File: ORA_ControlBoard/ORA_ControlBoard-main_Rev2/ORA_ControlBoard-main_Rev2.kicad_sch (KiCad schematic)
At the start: 66 parts, among them J1 SM04B-GHS-TB, J2 Conn_01x04_Pin, J3 USB_B_Micro, J4 12V, J5 SM04B-GHS-TB, J6 Conn_02x03_Top_Bottom, J7 Conn_01x05_Pin, J8 Conn_01x05_Pin, J9 Stack Light, Q1 BS170, Q3 BS170, Q5 BS170, SW1 Reset, U1 ATmega32U4-A, U2 MCP25625-x-SS, U5 NCP1117-5.0_SOT223, U6 IMU_MOUNT, Y1 8Mhz, Y2 16MHz

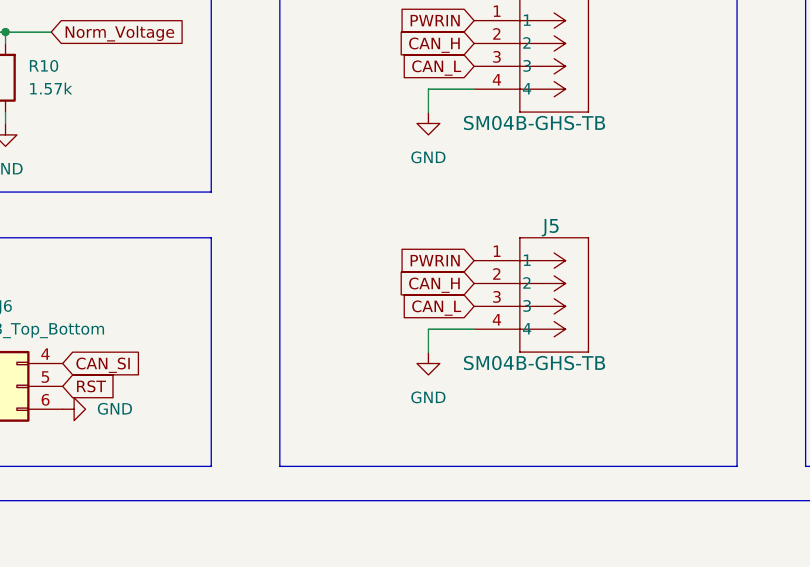
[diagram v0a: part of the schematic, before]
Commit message: Fixed Spring Cleaning
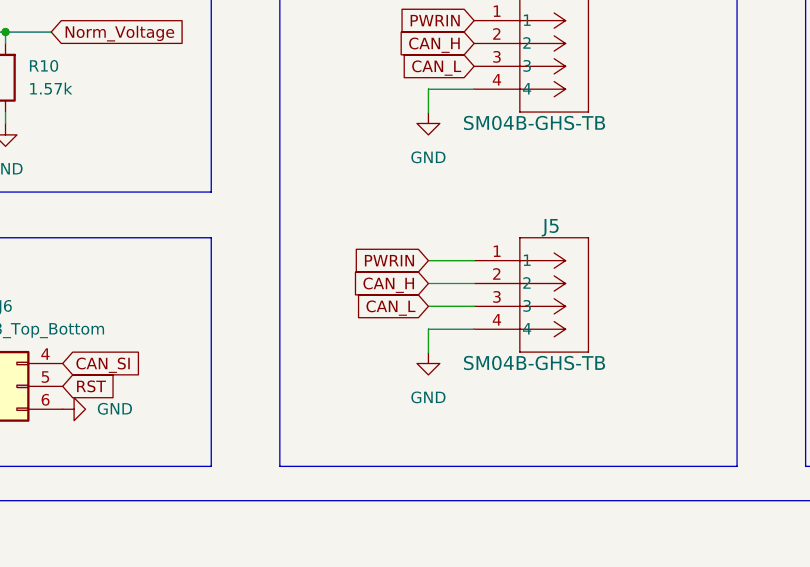
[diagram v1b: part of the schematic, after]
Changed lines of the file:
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@@
 	(wire
 		(pts
+			(xy 187.96 140.97) (xy 193.04 140.97)
+		)
+		(stroke
+			(width 0)
+			(type default)
+		)
+	)
+	(wire
+		(pts
 			(xy 287.02 101.6) (xy 280.67 101.6)
 		)
@@
 	(wire
 		(pts
+			(xy 187.96 138.43) (xy 193.04 138.43)
+		)
+		(stroke
+			(width 0)
+			(type default)
+		)
+	)
+	(wire
+		(pts
 			(xy 54.61 213.36) (xy 54.61 214.63)
 		)
@@
 	(wire
 		(pts
+			(xy 187.96 135.89) (xy 193.04 135.89)
+		)
+		(stroke
+			(width 0)
+			(type default)
+		)
+	)
+	(wire
+		(pts
 			(xy 266.7 78.74) (xy 262.89 78.74)
 		)
@@
 	(global_label "PWRIN"
 		(shape input)
-		(at 193.04 135.89 180)
+		(at 187.96 135.89 180)
 		(fields_autoplaced yes)
 		(effects
@@
 		)
 		(property "Intersheetrefs" "${INTERSHEET_REFS}"
-			(at 184.1281 135.89 0)
+			(at 179.0481 135.89 0)
 			(effects
 				(font
@@
 	(global_label "CAN_L"
 		(shape input)
-		(at 193.04 140.97 180)
+		(at 187.96 140.97 180)
 		(fields_autoplaced yes)
 		(effects
@@
 		)
 		(property "Intersheetrefs" "${INTERSHEET_REFS}"
-			(at 184.37 140.97 0)
+			(at 179.29 140.97 0)
 			(effects
 				(font
@@
 	(global_label "CAN_H"
 		(shape input)
-		(at 193.04 138.43 180)
+		(at 187.96 138.43 180)
 		(fields_autoplaced yes)
 		(effects
@@
 		)
 		(property "Intersheetrefs" "${INTERSHEET_REFS}"
-			(at 184.0676 138.43 0)
+			(at 178.9876 138.43 0)
 			(effects
 				(font

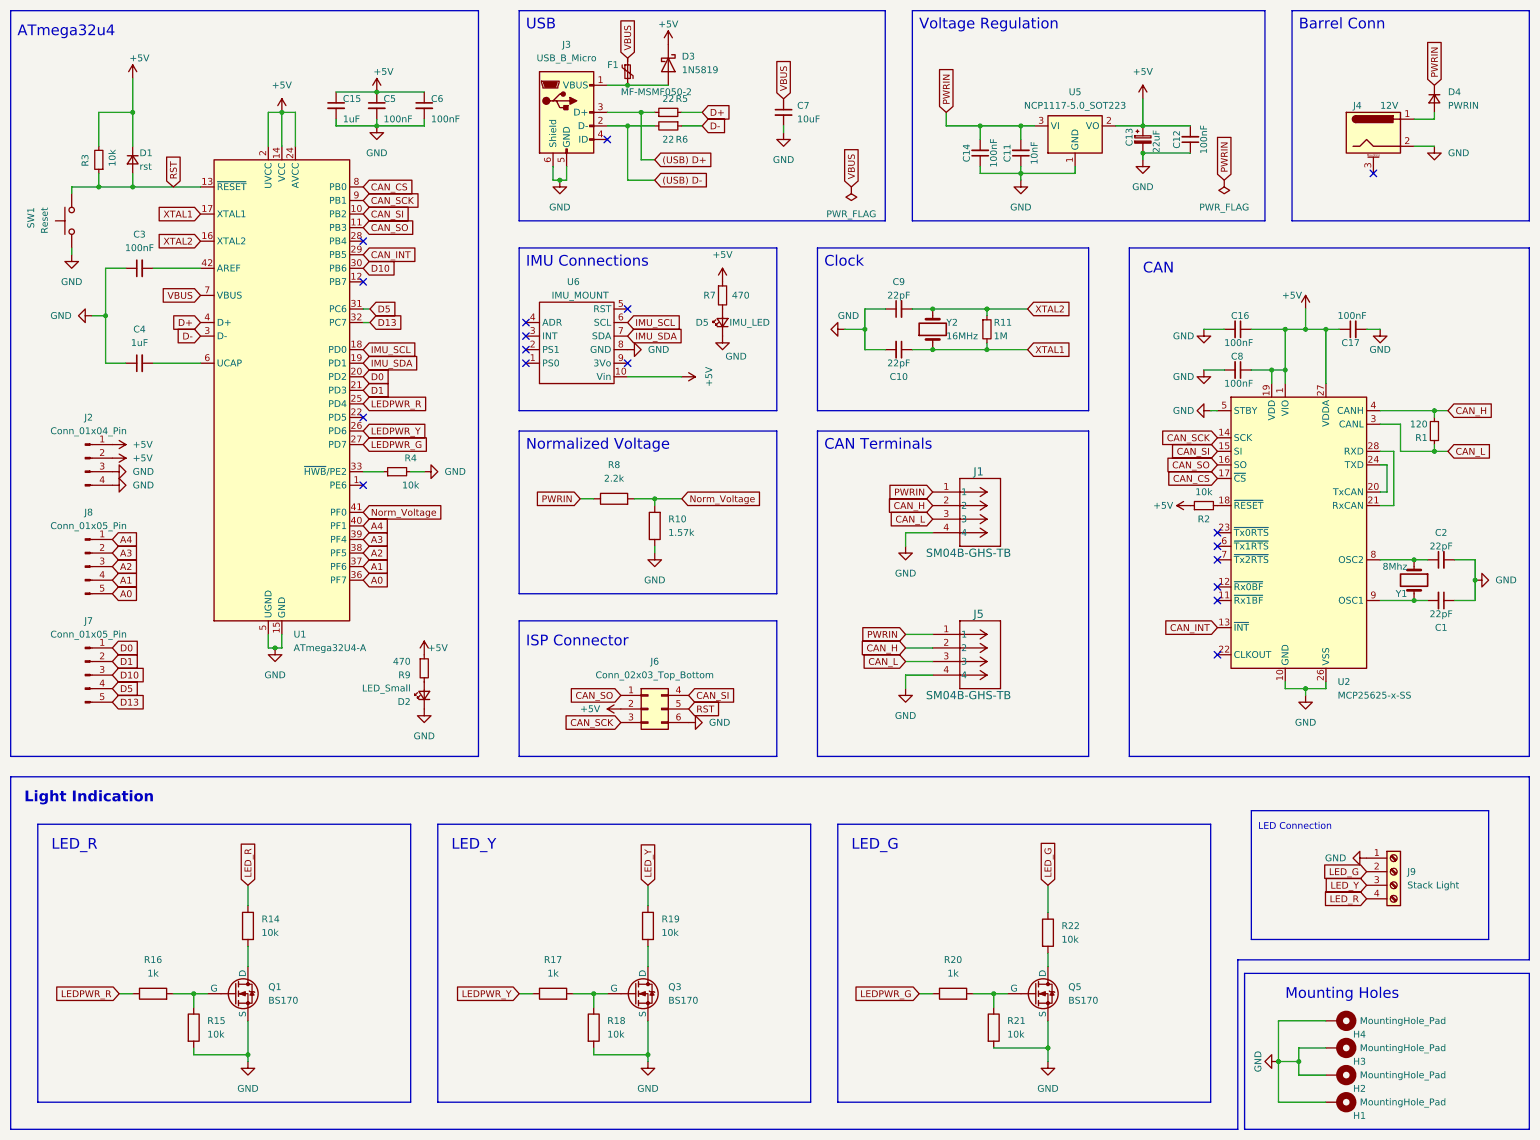
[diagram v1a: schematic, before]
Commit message: "Final" Rev 2 changes
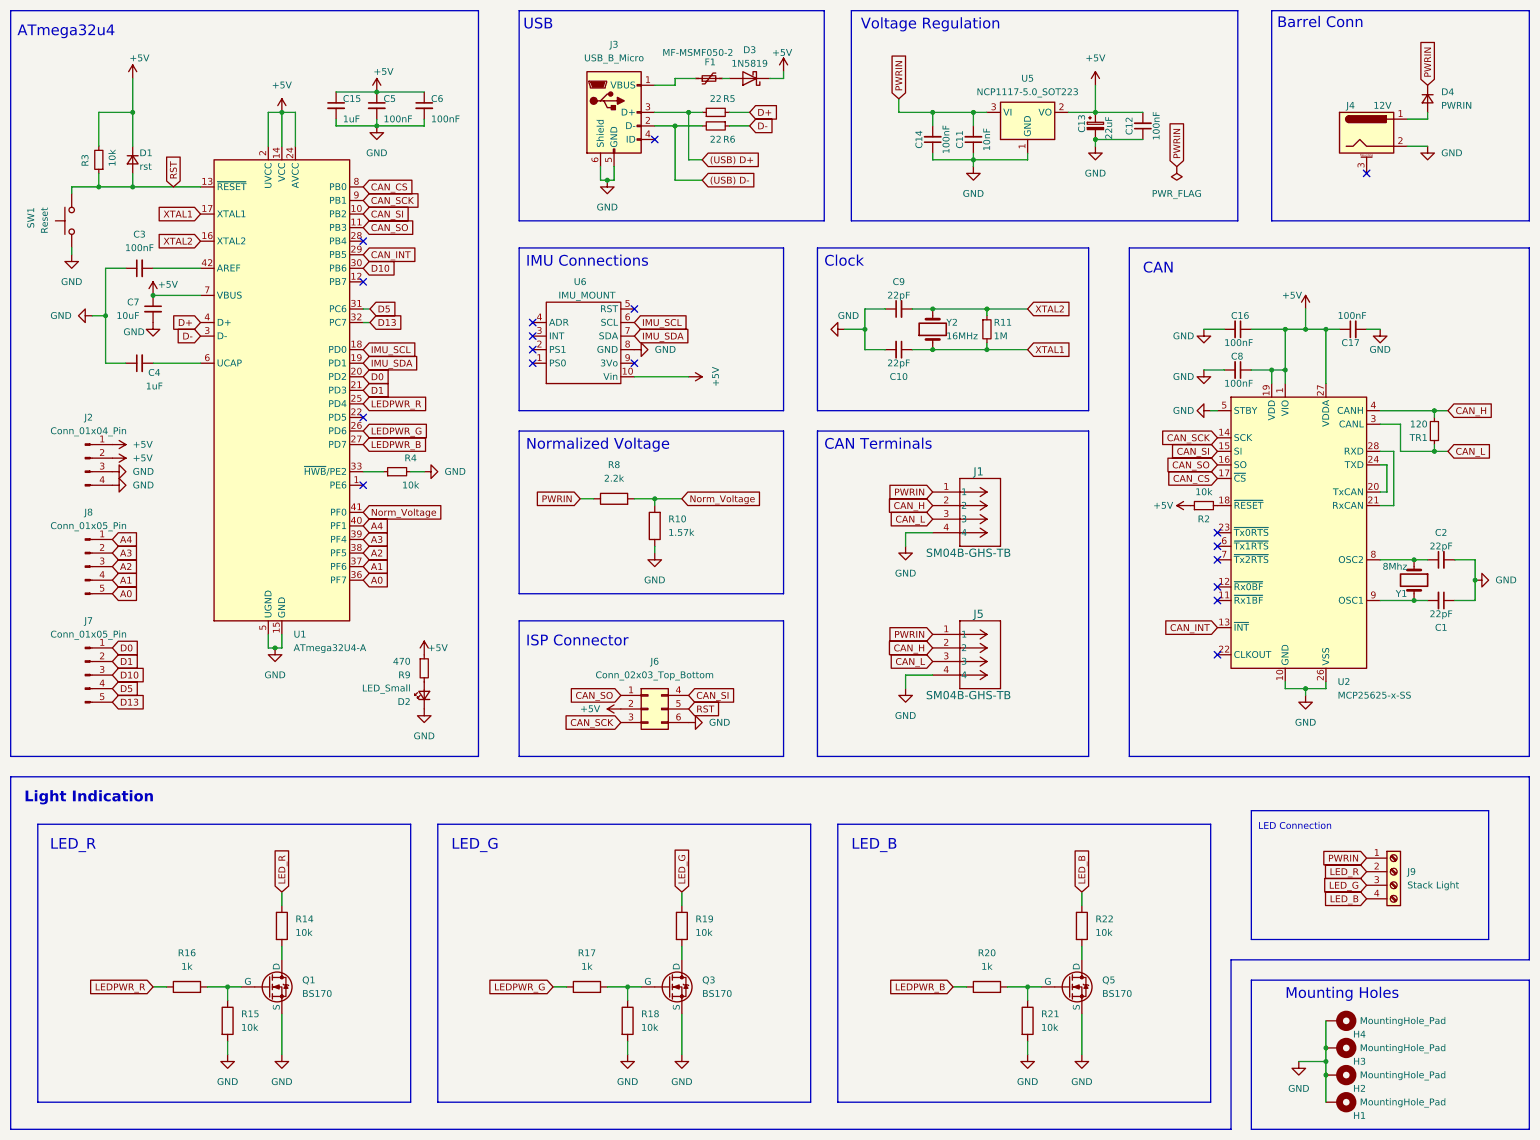
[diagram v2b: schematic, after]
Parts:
- removed D5: IMU_LED, LED_SMD:LED_0805_2012Metric_Pad1.15x1.40mm_HandSolder, symbol Device:LED_Small
- removed R7: 470, Resistor_SMD:R_0805_2012Metric_Pad1.20x1.40mm_HandSolder, symbol Device:R_Small
- J3: footprint Connector_USB:USB_Micro-B_Amphenol_10118193-0002LF_Horizontal -> AdditionalParts:AMPHENOL_10118192-0002LF
- renumbered R1 to TR1
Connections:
- net LEDPWR_Y is gone; now on net LEDPWR_G: R17.1, U1.26 (PD6)
- net LED_Y is gone; now on net LED_G: J9.3 (Pin_3), R19.1
- net +5V: now also C7.1, U1.7 (VBUS)
- net GND: no longer J9.1 (Pin_1)
- net LEDPWR_G: no longer R20.1, U1.27 (PD7)
- net LED_G: no longer J9.2 (Pin_2), R22.1
- net LED_R: now also J9.2 (Pin_2); no longer J9.4 (Pin_4)
- net PWRIN: now also J9.1 (Pin_1)
- net at D3.2 (A), F1.2: no longer J3.1 (VBUS)
- removed net VBUS: C7.1, F1.1, U1.7 (VBUS)
- new net: F1.1, J3.1 (VBUS)
- new net LEDPWR_B: R20.1, U1.27 (PD7)
- new net LED_B: J9.4 (Pin_4), R22.1
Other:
- note added: "LED_B"
- note removed: "LED_Y"
- moved on the sheet: C11, C12, C13, C14, D3, D4, J3, J4, Q1, Q3, Q5, R14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
